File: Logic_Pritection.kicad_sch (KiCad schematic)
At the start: 11 parts

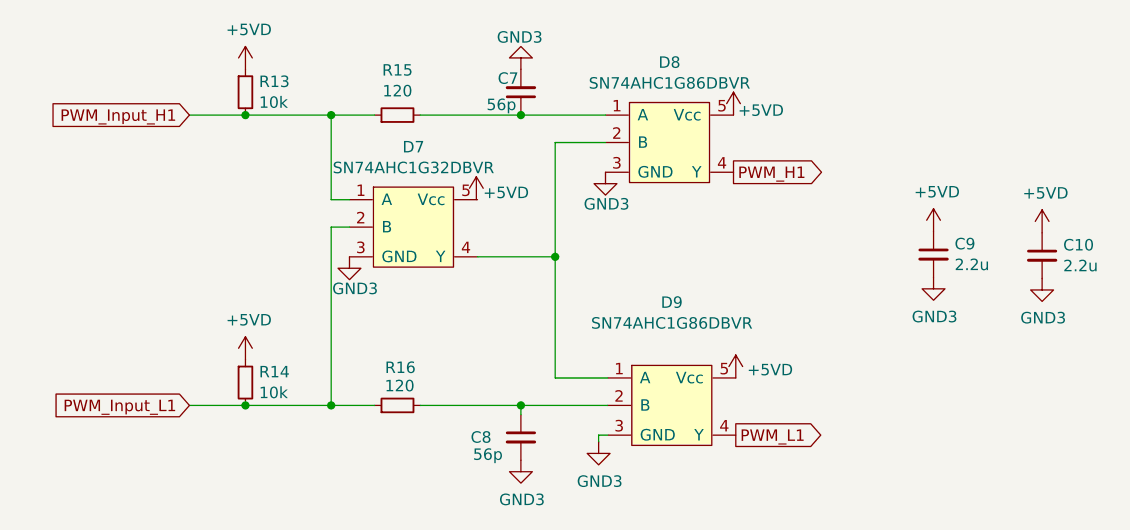
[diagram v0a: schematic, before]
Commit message: Одна стойка
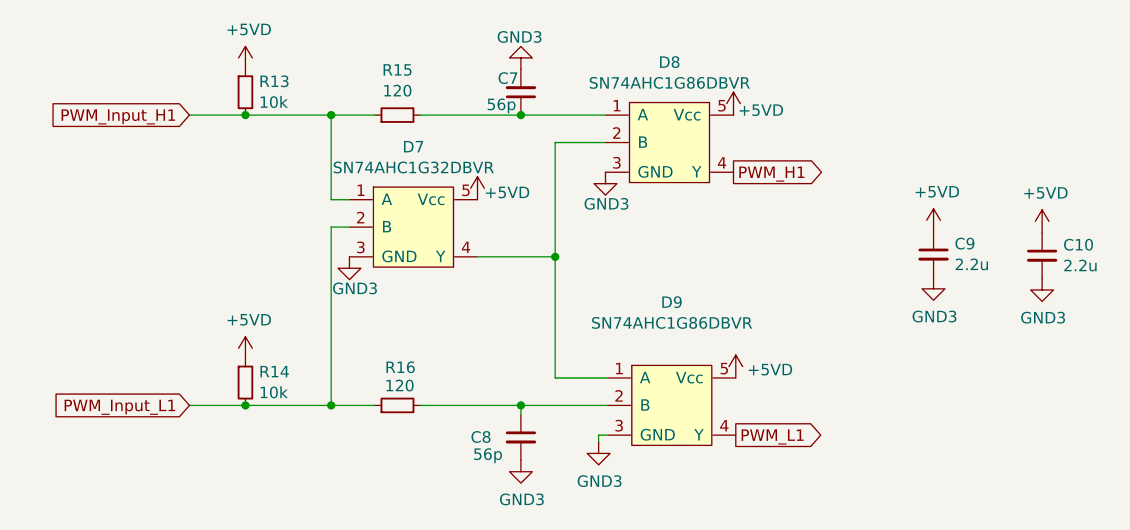
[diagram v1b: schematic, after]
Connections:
- net +5VD: now also D7.5 (Vcc)
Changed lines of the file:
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@@
     (pin "1")
   )
-  (symbol (lib_id "power:+5VD") (at 135.255 79.502 0) (unit 1)
+  (symbol (lib_id "power:+5VD") (at 135.382 79.502 0) (unit 1)
     (in_bom yes) (on_board yes)
-    (property "Reference" "#PWR018" (id 0) (at 135.255 83.312 0)
+    (property "Reference" "#PWR018" (id 0) (at 135.382 83.312 0)
       (effects (font (size 1.27 1.27)) hide)
     )
-    (property "Value" "+5VD" (id 1) (at 138.557 78.74 0))
-    (property "Footprint" "" (id 2) (at 135.255 79.502 0)
+    (property "Value" "+5VD" (id 1) (at 138.684 78.74 0))
+    (property "Footprint" "" (id 2) (at 135.382 79.502 0)
       (effects (font (size 1.27 1.27)) hide)
     )
-    (property "Datasheet" "" (id 3) (at 135.255 79.502 0)
+    (property "Datasheet" "" (id 3) (at 135.382 79.502 0)
       (effects (font (size 1.27 1.27)) hide)
     )
